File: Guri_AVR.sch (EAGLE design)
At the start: 66 parts, among them IC1 7805, IC2 MEGA8-P, IC3 74LS74N, Q1 BC337, Q2 BC556, Q3 IRGB14C40L, Q5 BC548, X1 16.0

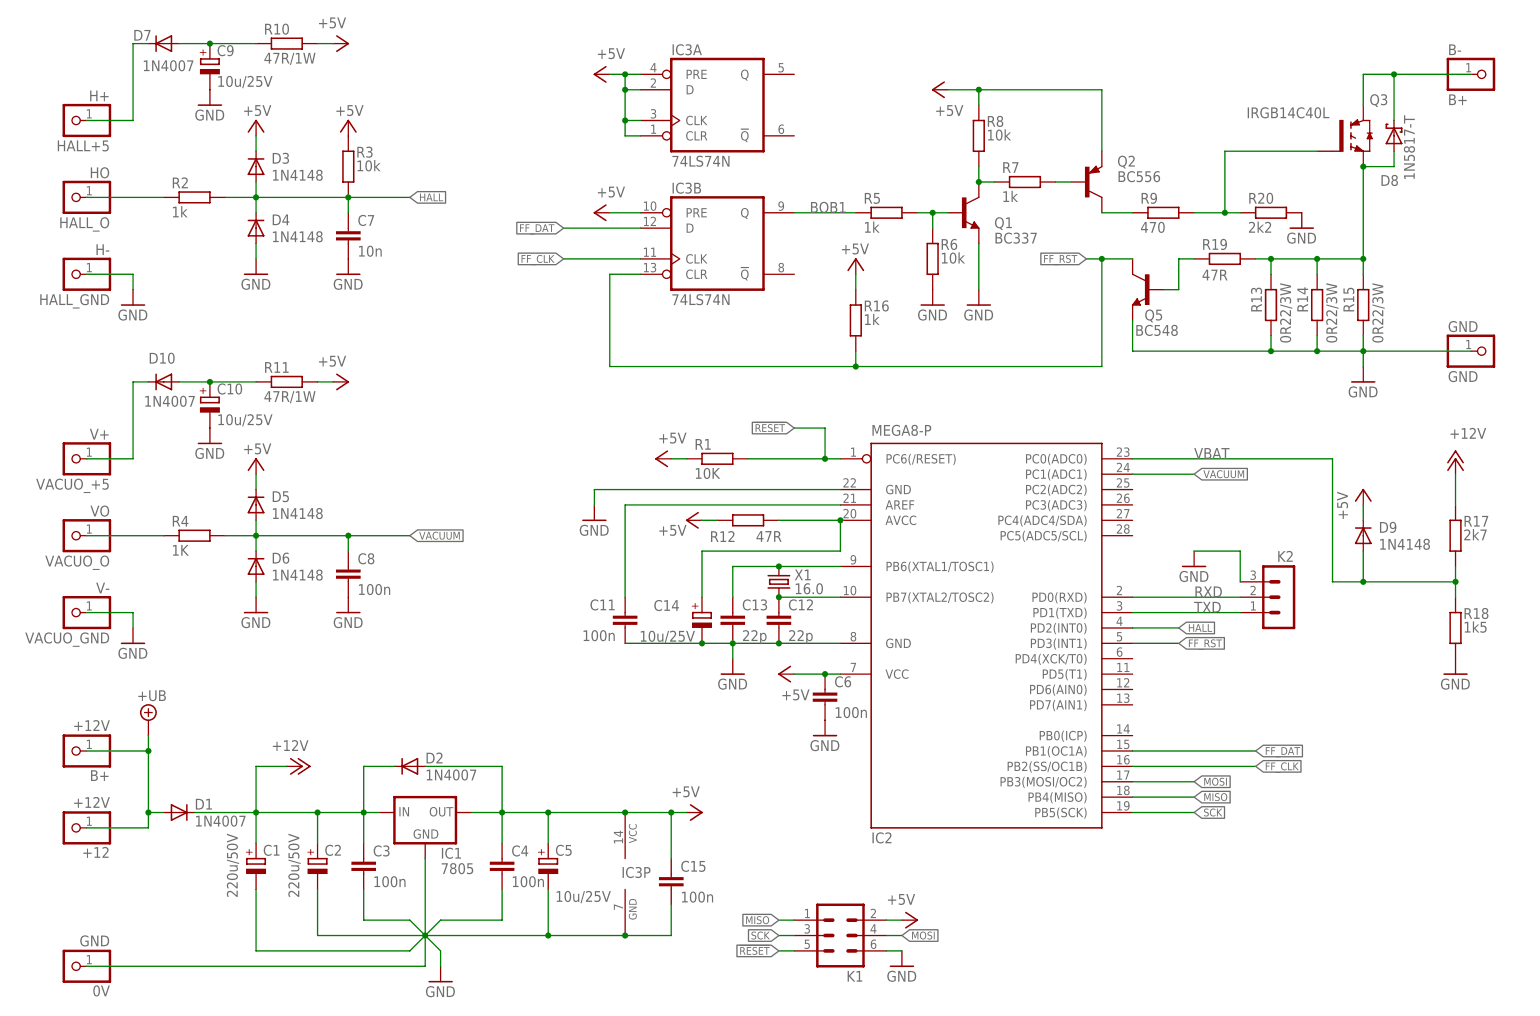
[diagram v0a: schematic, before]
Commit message: New layout for preliminary board
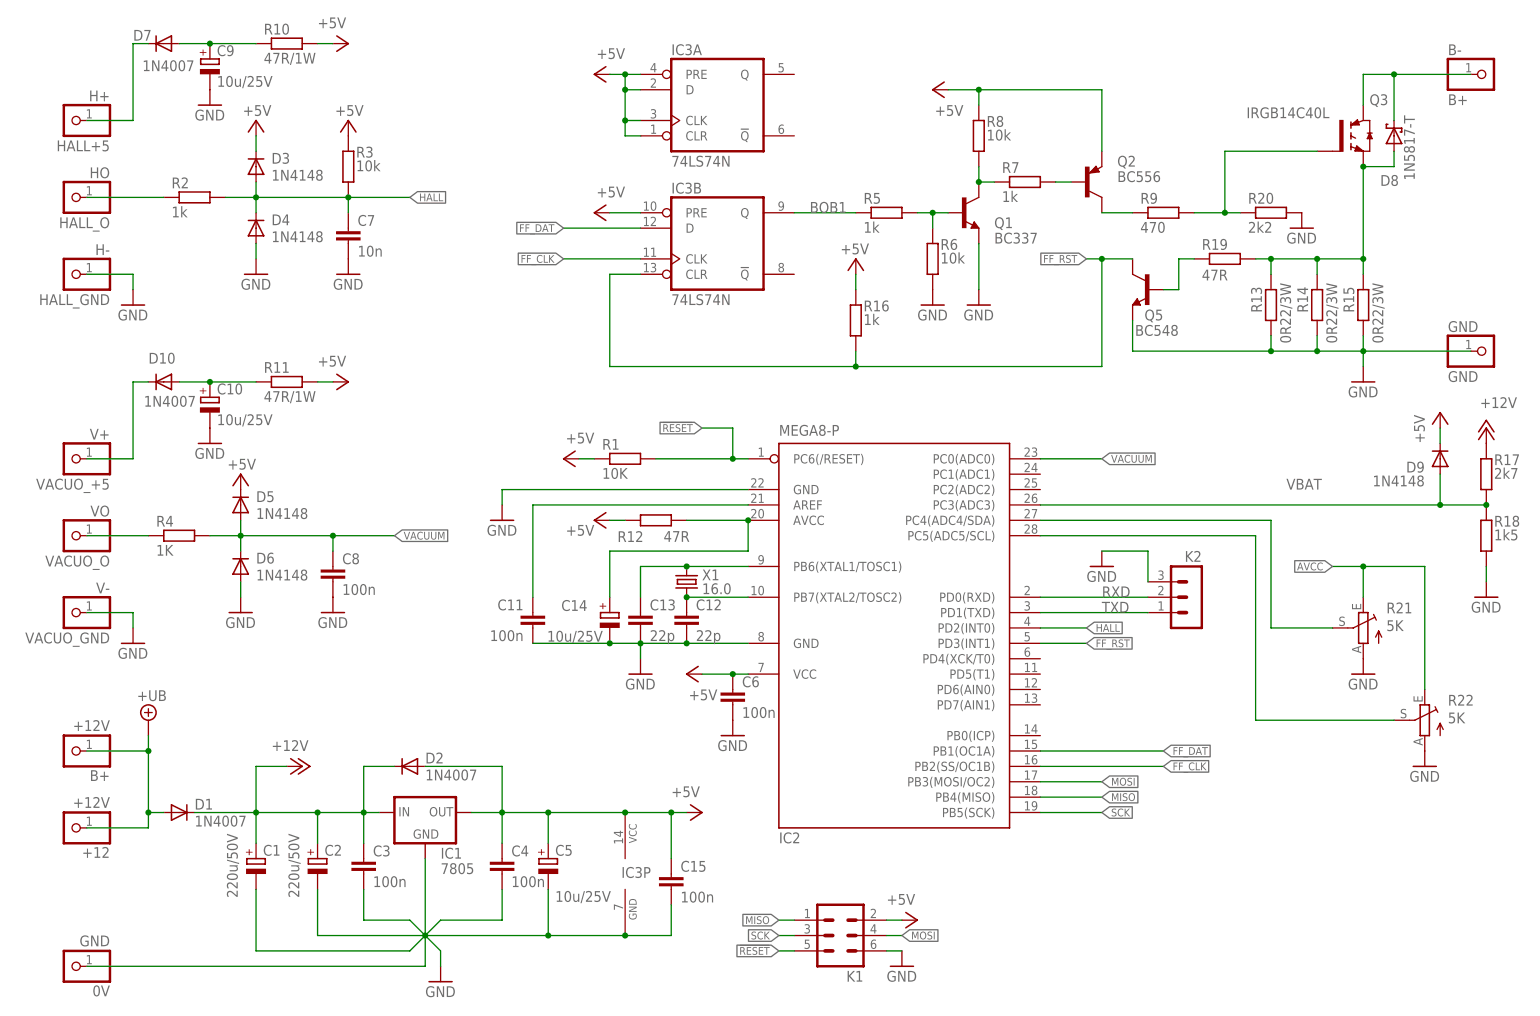
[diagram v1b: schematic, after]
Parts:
- added R21, R22: 5K, pot:TRIM_EU-ECP10P
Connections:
- new net N$16: IC2.PC4(ADC4/SDA), R21.S
- new net N$17: IC2.PC5(ADC5/SCL), R22.S
- net AVCC: now also R21.E, R22.E
- net GND: now also R21.A, R22.A
- net VACUUM: now also IC2.PC0(ADC0); no longer IC2.PC1(ADC1)
- net VBAT: now also IC2.PC3(ADC3); no longer IC2.PC0(ADC0)
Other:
- moved on the sheet: C11, C12, C13, C14, C6, C8, D5, D6, D9, IC2, K2, R1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
